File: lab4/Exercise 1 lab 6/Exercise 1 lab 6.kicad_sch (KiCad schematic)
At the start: 6 parts, among them SW1 SW_SPDT

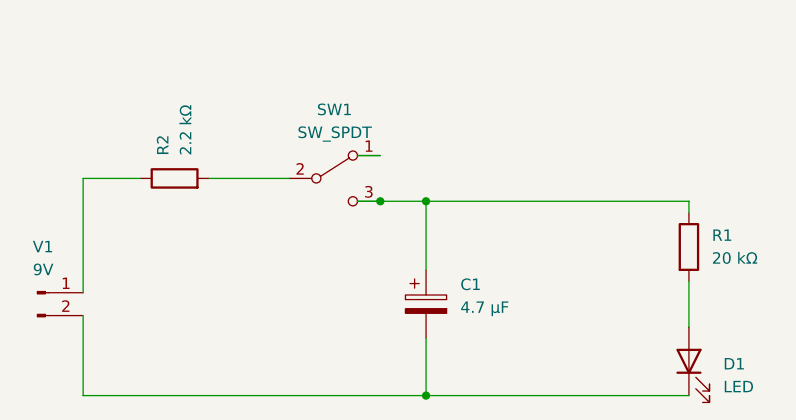
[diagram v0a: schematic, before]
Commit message: lab 6
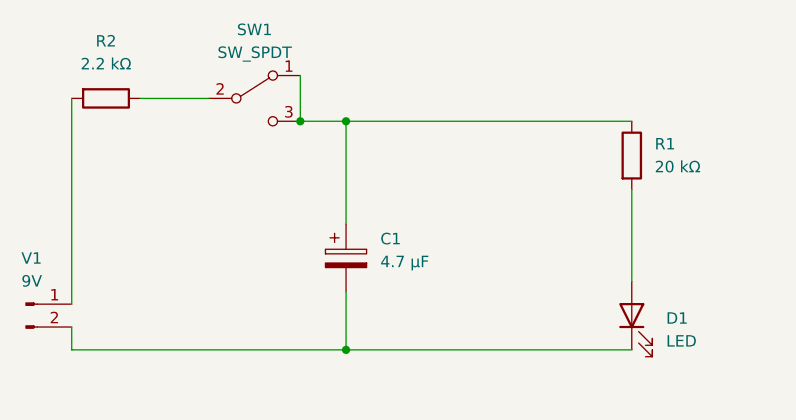
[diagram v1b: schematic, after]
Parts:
- C1: value 4.7 µF -> 4.7 μF; footprint (none) -> Capacitor_THT:C_Radial_D5.0mm_H5.0mm_P2.00mm
- D1: footprint (none) -> LED_THT:LED_D5.0mm
- R1, R2: footprint (none) -> Resistor_THT:R_Axial_DIN0516_L15.5mm_D5.0mm_P20.32mm_Horizontal
- SW1: footprint (none) -> Button_Switch_THT:SW_E-Switch_EG1224_SPDT_Angled
- V1: footprint (none) -> Connector_JST:JST_PH_B2B-PH-K_1x02_P2.00mm_Vertical
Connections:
- net at SW1.1 (A): now also C1.1, R1.1, SW1.3 (C)
- net at SW1.2 (B): now also R2.1; no longer R2.2
- net at V1.1 (Pin_1): now also R2.2; no longer R2.1
